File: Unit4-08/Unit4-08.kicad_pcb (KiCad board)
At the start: 2 copper layers, 13 parts, among them SW1 SW_Push, SW2 SW_Push, U1 74LS08, U2 74LS08

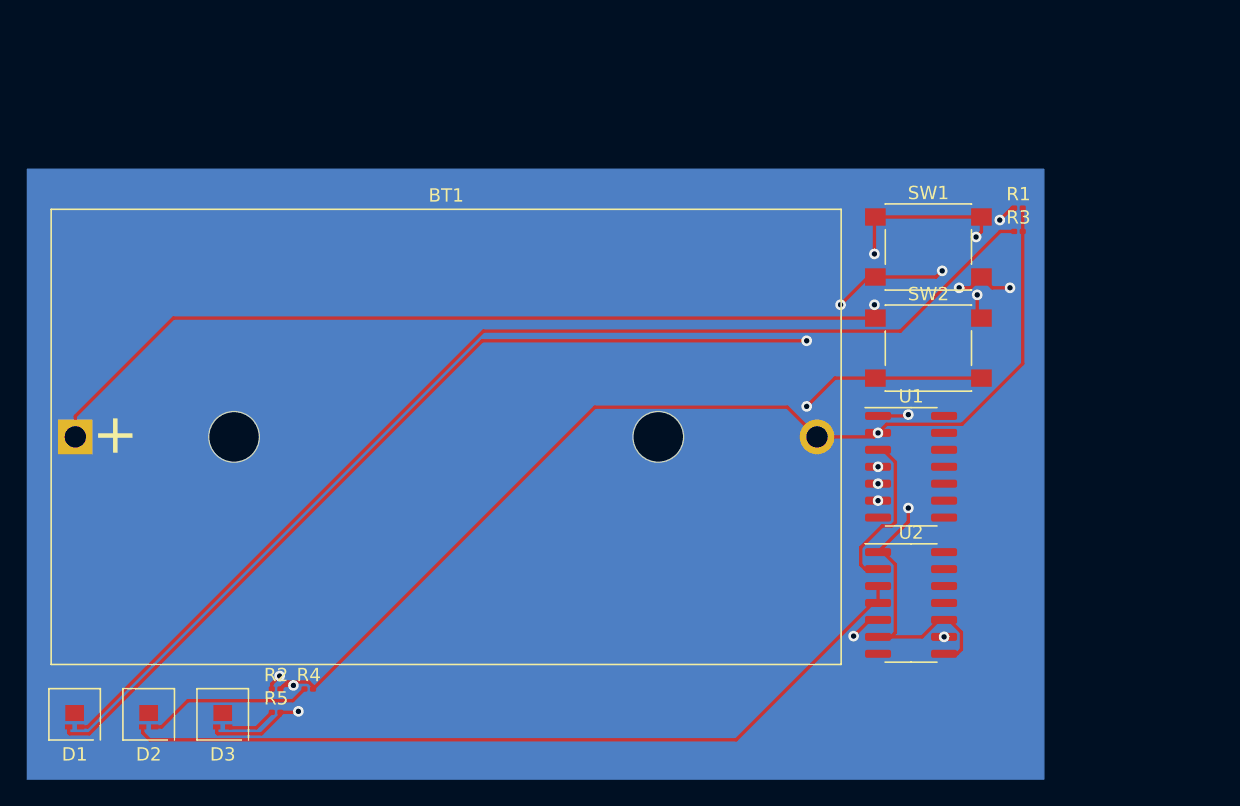
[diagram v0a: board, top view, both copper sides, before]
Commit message: Updated PCB
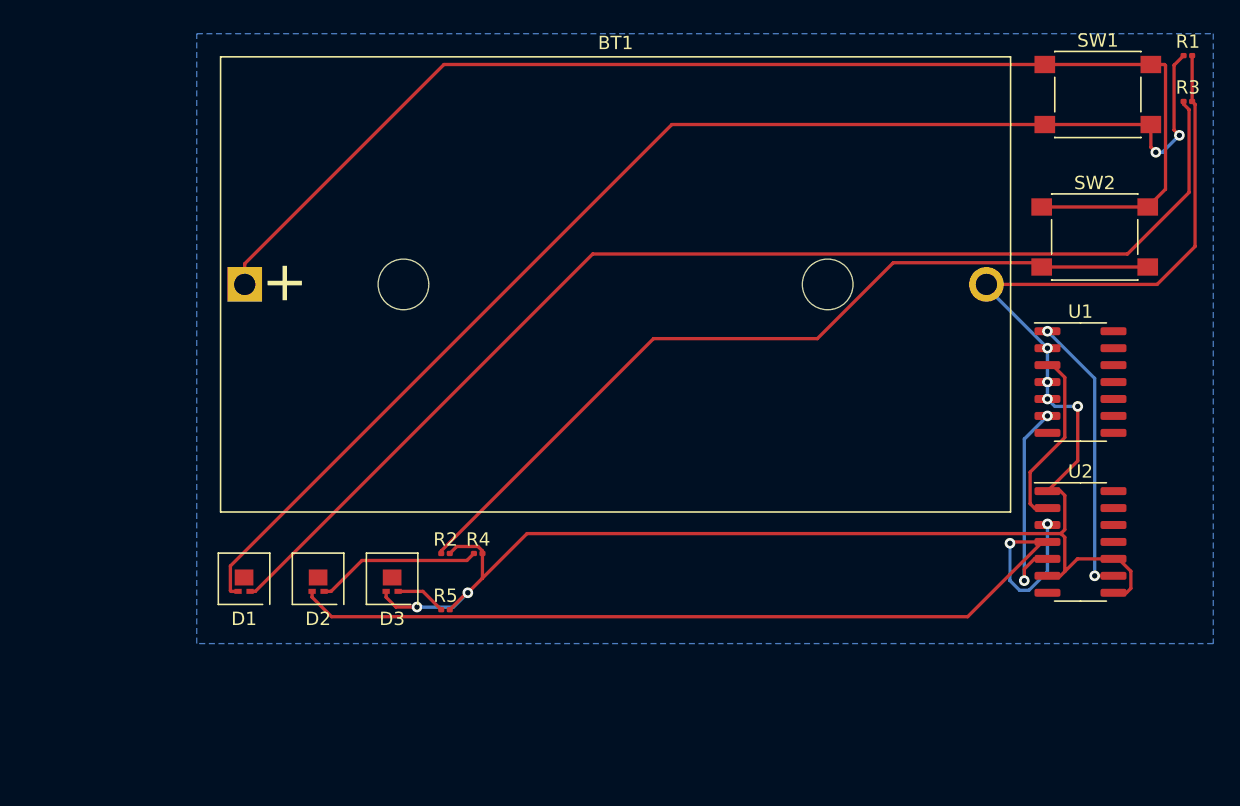
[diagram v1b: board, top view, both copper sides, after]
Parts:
- moved BT1 17.1 mm to (114.1, 93.7)
- moved R1 17.1 mm to (184.8, 76.6)
- moved SW1 17.1 mm to (178.0, 79.5)
- moved R4 16.3 mm to (131.6, 113.9)
- moved D2 16.3 mm to (119.6, 116.2)
- moved D3 16.3 mm to (125.1, 116.2)
- moved R2 16.3 mm to (129.1, 113.9)
- moved D1 16.3 mm to (114.0, 116.2)
- moved R3 16.0 mm to (184.8, 80.0)
- moved SW2 15.0 mm to (177.8, 90.2)
- moved R5 14.8 mm to (129.1, 118.1)
- moved U1 14.2 mm to (176.7, 101.0)
- moved U2 13.5 mm to (176.7, 113.0)
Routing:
- net Net-(D2-Pad2): track 61.3 -> 71.4 mm, vias 0 -> 2
- net Net-(BT1-Pad2): track 119.6 -> 129.1 mm, vias 6 -> 7
- net Net-(BT1-Pad1): track 88.1 -> 95.9 mm, vias 4 -> 0
- net Net-(D1-Pad1): track 85.4 -> 89.8 mm
- net Net-(U1-Pad6): track 13.3 -> 16.0 mm
- net Net-(D1-Pad2): track 93.5 -> 96.1 mm, vias 6 -> 2
- net Net-(U1-Pad3): track 12.3 -> 13.7 mm
- net Net-(U1-Pad1): track 20.1 -> 21.2 mm
- net Net-(R2-Pad1): track 63.1 -> 62.2 mm, vias 2 -> 0
- added copper zone on B.Cu, net (none)
